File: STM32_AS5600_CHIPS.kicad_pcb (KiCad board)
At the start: 2 copper layers, 29.6 x 37.2 mm, 39 parts, among them IC1 AS5600-ASOT, J1 Conn_01x04_Pin, J3 Conn_01x07_Pin, J4 USB4105-GF-A-120, U1 STM32F103C8Tx, U2 AMS1117-3.3, Y2 Crystal

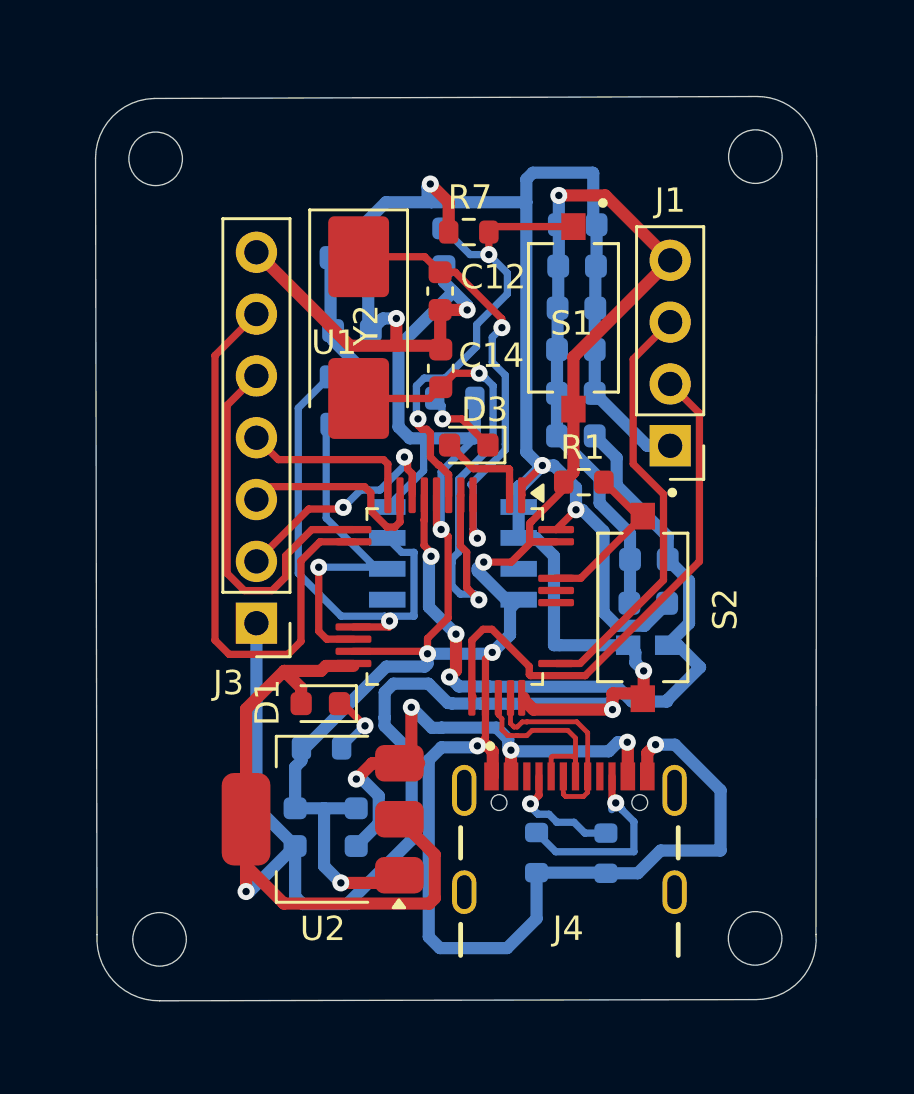
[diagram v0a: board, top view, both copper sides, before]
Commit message: Add files via upload
2nd Commit
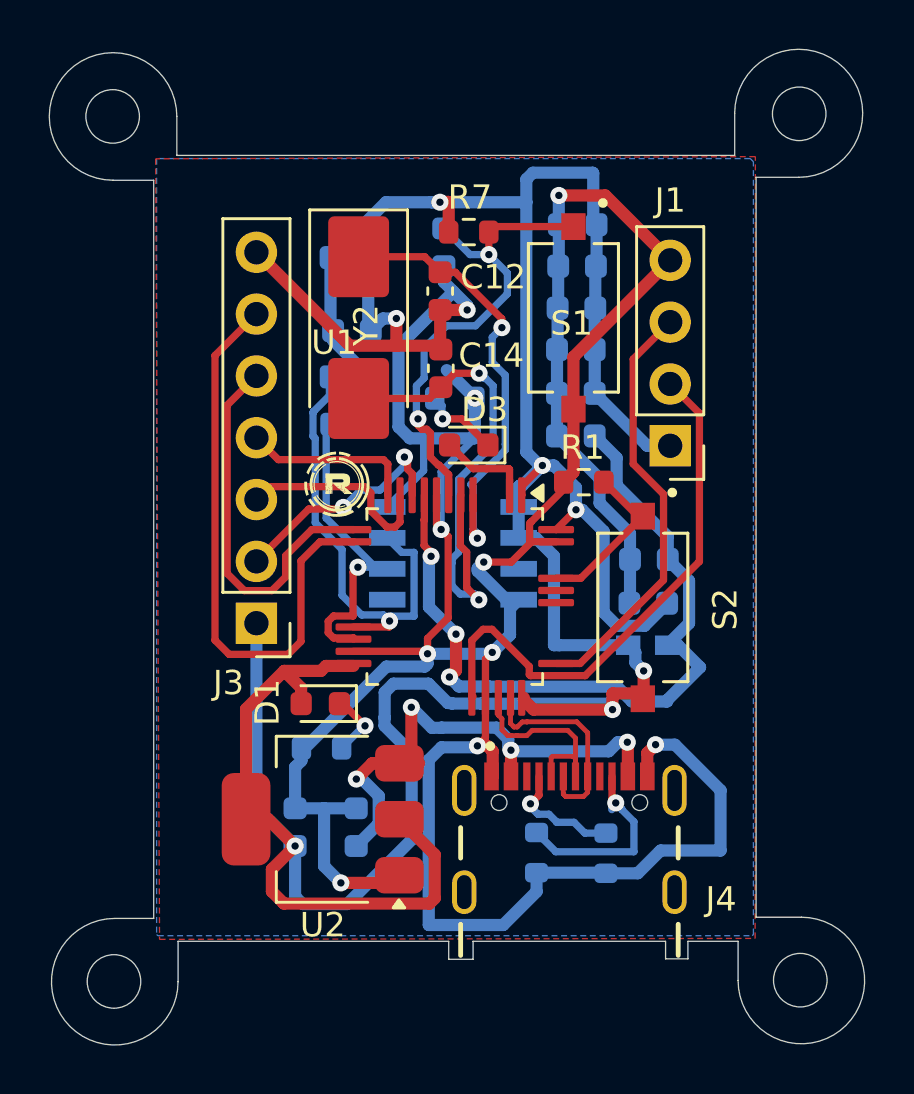
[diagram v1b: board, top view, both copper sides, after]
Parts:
- added G***: LOGO, LOGO, F.Cu at (183.5, 75.4)
- R7: value R -> 10k
- moved H4 2.55 mm to (174.3, 95.8)
- moved H3 2.53 mm to (202.5, 95.7)
- moved H2 2.52 mm to (202.5, 60.1)
- moved H1 2.48 mm to (174.2, 60.2)
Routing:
- net +3.3V: track 147.3 -> 141.8 mm
- net /I2C_SCL: track 20.0 -> 19.0 mm
- net /I2C_SDA: track 14.9 -> 13.9 mm
- net GND: vias 10 -> 11
- added copper zone on B.Cu, net GND
- added copper zone on F.Cu, net GND
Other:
- board size 29.6 x 37.2 mm -> 33.5 x 40.9 mm
